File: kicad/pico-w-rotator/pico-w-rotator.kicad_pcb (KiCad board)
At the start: 2 copper layers, 86.4 x 76.2 mm, 163 parts, among them J1 DB9_Male, SW1 Mode Button, U1 PicoW, U2 MAX3232, U3 LM7805_TO220

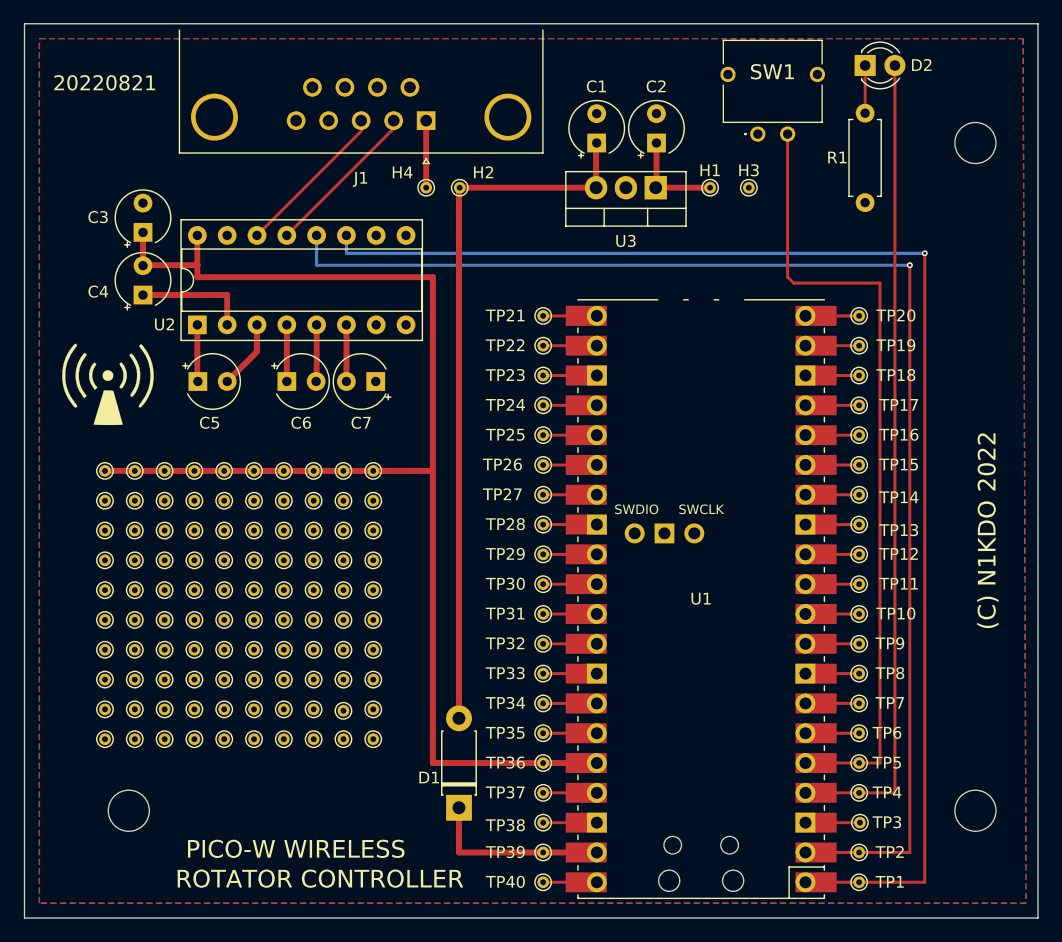
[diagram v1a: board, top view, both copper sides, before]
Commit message: pcb measured, checked
sent out to oshpark!
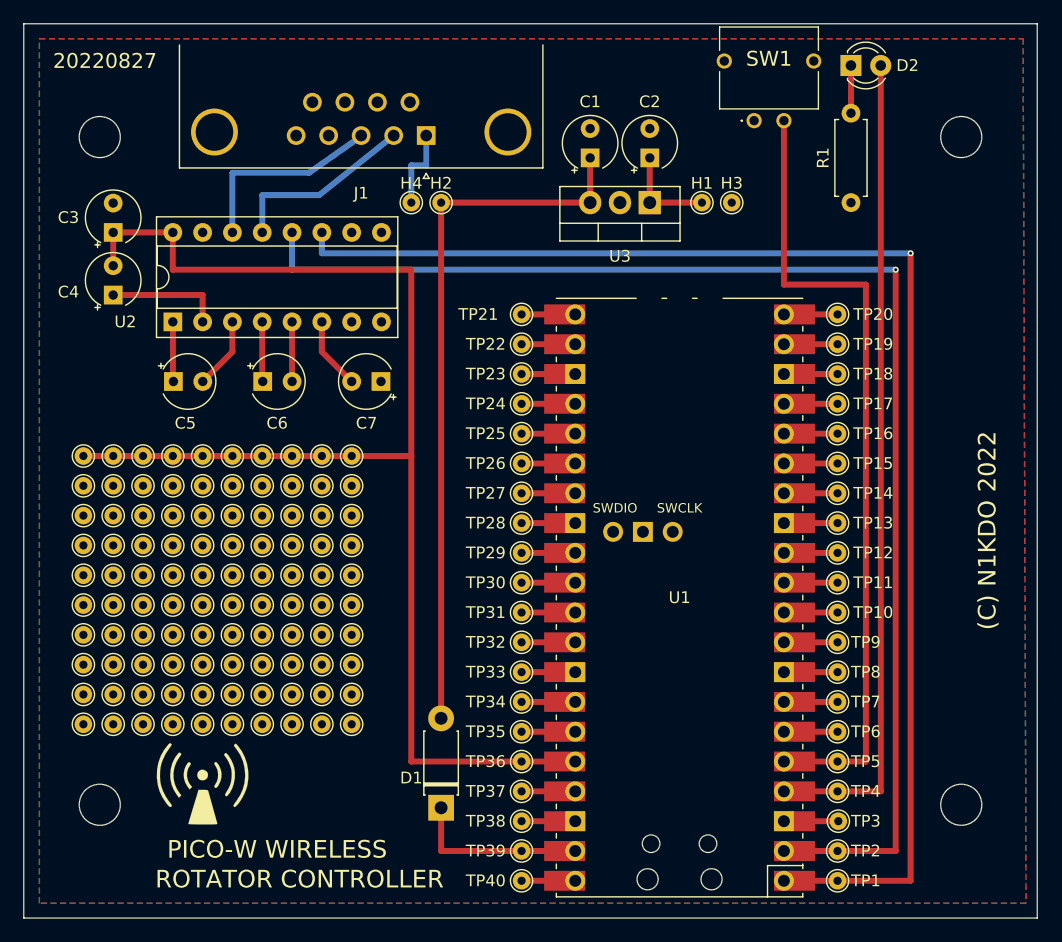
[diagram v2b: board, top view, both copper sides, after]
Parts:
- added H6: MountingHole, MountingHole:MountingHole_3.5mm, F.Cu at (31.9, 35.1)
- GH1, GH10, GH100, GH11, GH12, GH13, GH14, GH15, GH16, GH17, GH18, GH19, GH2, GH20, GH21, GH22, GH23, GH24, GH25, GH26, GH27, GH28, GH29, GH3, GH30, GH31, GH32, GH33, GH34, GH35, GH36, GH37, GH38, GH39, GH4, GH40, GH41, GH42, GH43, GH44, GH45, GH46, GH47, GH48, GH49, GH5, GH50, GH51, GH52, GH53, GH54, GH55, GH56, GH57, GH58, GH59, GH6, GH60, GH61, GH62, GH63, GH64, GH65, GH66, GH67, GH68, GH69, GH7, GH70, GH71, GH72, GH73, GH74, GH75, GH76, GH77, GH78, GH79, GH8, GH80, GH81, GH82, GH83, GH84, GH85, GH86, GH87, GH88, GH89, GH9, GH90, GH91, GH92, GH93, GH94, GH95, GH96, GH97, GH98, GH99, H1, H2, H3, H4, TP1, TP10, TP11, TP12, TP13, TP14, TP15, TP16, TP17, TP18, TP19, TP2, TP20, TP21, TP22, TP23, TP24, TP25, TP26, TP27, TP28, TP29, TP3, TP30, TP31, TP32, TP33, TP34, TP35, TP36, TP37, TP38, TP39, TP4, TP40, TP5, TP6, TP7, TP8, TP9: footprint TestPoint:TestPoint_THTPad_D1.0mm_Drill0.5mm -> TestPoint:TestPoint_THTPad_D1.5mm_Drill0.7mm
- moved G1 35.0 mm to (40.6, 90.2)
- moved C3 2.54 mm to (33.0, 43.2)
- moved C4 2.54 mm to (33.0, 48.5)
- moved H7 2.53 mm to (31.9, 91.9)
- moved GH89 2.31 mm to (50.8, 82.5)
- moved GH52 2.24 mm to (43.2, 64.8)
- moved GH54 2.24 mm to (43.2, 69.8)
- moved GH62 2.24 mm to (45.7, 64.8)
- moved GH64 2.24 mm to (45.7, 69.8)
- moved GH72 2.24 mm to (48.3, 64.8)
- moved GH74 2.24 mm to (48.3, 69.8)
- moved GH82 2.24 mm to (50.8, 64.8)
- moved GH84 2.24 mm to (50.8, 69.8)
- moved GH2 2.24 mm to (30.5, 64.8)
- moved GH4 2.24 mm to (30.5, 69.8)
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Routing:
- net Net-(J1-Pad3): track 13.9 -> 17.1 mm
- net Net-(J1-Pad2): track 14.0 -> 16.2 mm
- net Net-(D1-Pad1): track 15.6 -> 17.1 mm
- net TX: track 114.6 -> 116.0 mm
- net RX: track 112.0 -> 113.4 mm
- net Net-(C7-Pad2): track 4.83 -> 6.13 mm
- net +3.3V: track 114.1 -> 115.2 mm
- net Net-(SW1-Pad2): track 67.5 -> 68.6 mm
- net Net-(H4-Pad1): track 6.10 -> 6.98 mm
- net Net-(C4-Pad1): track 9.40 -> 10.2 mm
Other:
- board text added: "20220827"
- board text removed: "20220821"
